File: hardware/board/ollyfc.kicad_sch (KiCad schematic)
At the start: 84 parts, among them CN1 20021521-00010T1LF, J1 Conn_01x04, J3 Conn_01x07, J4 Conn_01x06, Q2 MMBT3904, Q3 MMBT3904, SW1 MODE1, SW2 SW_Push, SW5 MODE1, U3 STM32F411RETx, U6 W25Q128JVS, X1 X322516MLB4SI

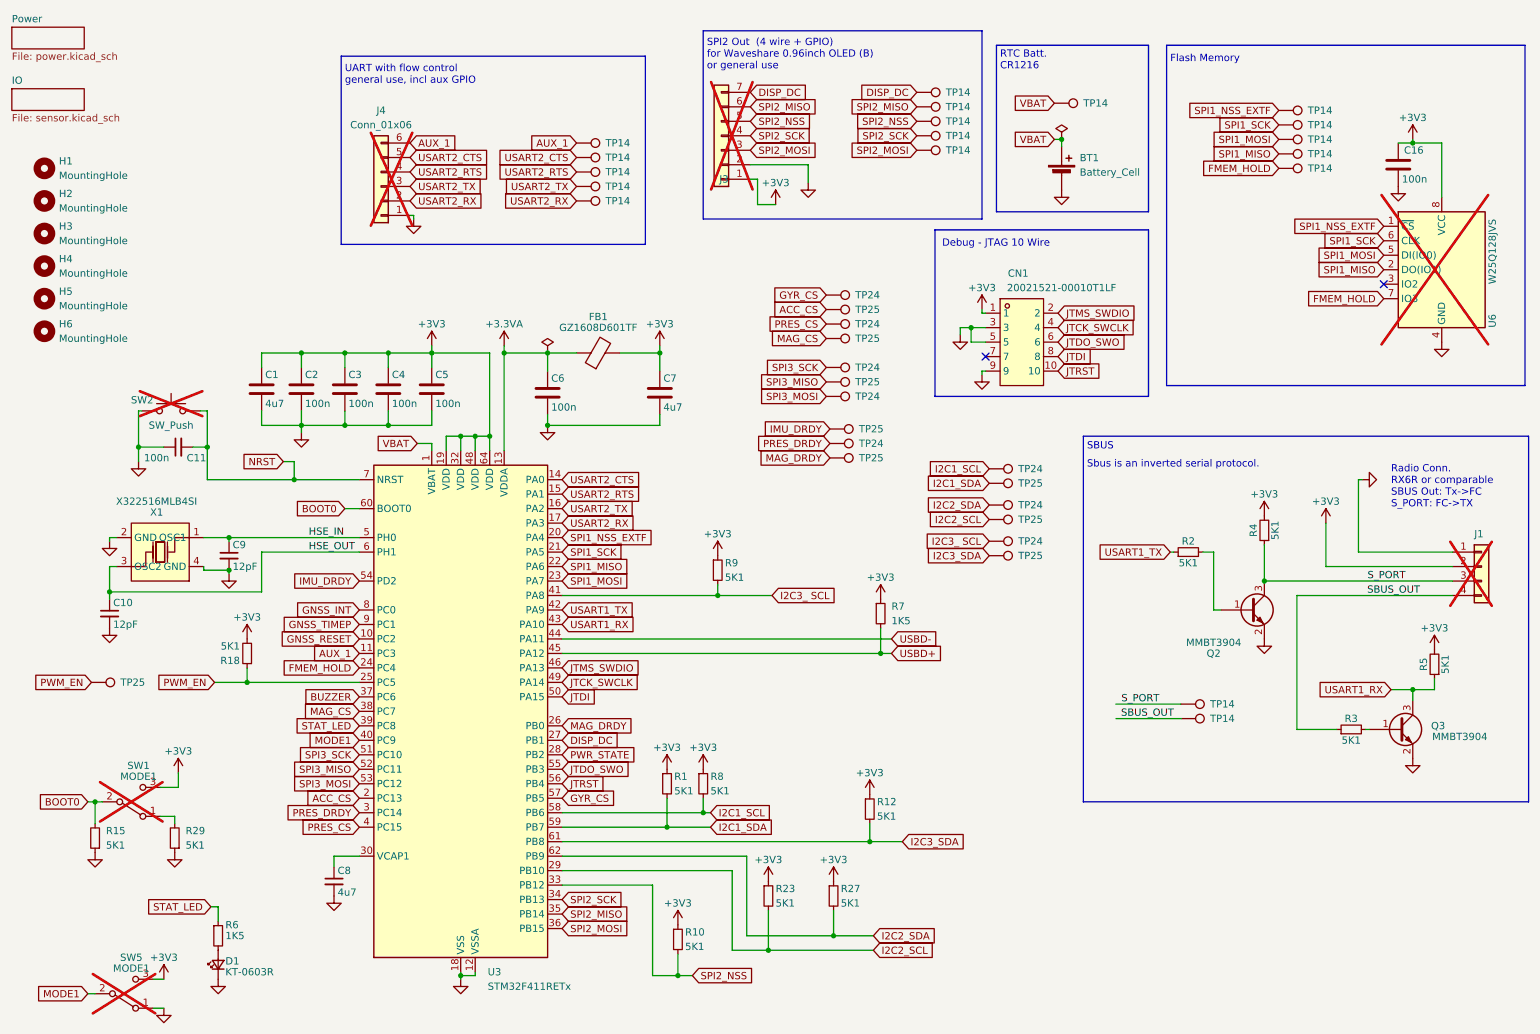
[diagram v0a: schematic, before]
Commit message: dead-end board files
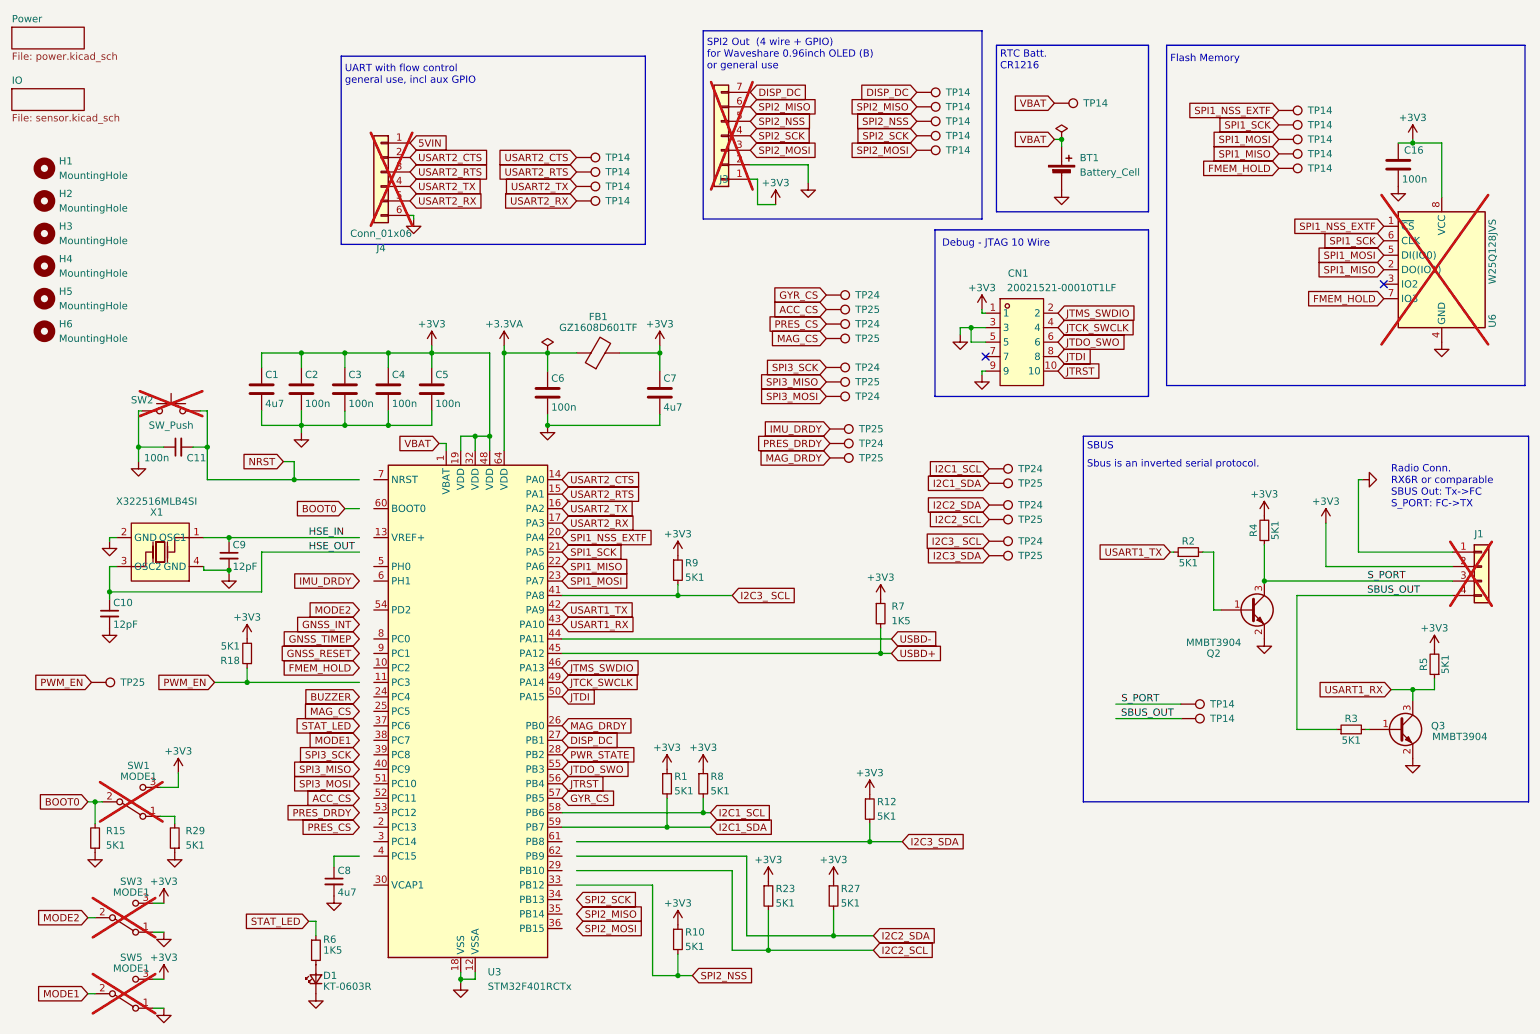
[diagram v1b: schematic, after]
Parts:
- removed TP14: TestPoint, TestPoint:TestPoint_Pad_D1.0mm, symbol Connector:TestPoint
- removed U3: STM32F411RETx, Package_QFP:LQFP-64_10x10mm_P0.5mm, symbol MCU_ST_STM32F4:STM32F411RETx
- added SW3: MODE1, Button_Switch_SMD:SW_SPDT_PCM12, symbol Switch:SW_SPDT
- added U3: STM32F401RCTx, Package_QFP:LQFP-64_10x10mm_P0.5mm, symbol MCU_ST_STM32F4:STM32F401RCTx
- J1: footprint Connector_JST:JST_PH_B4B-PH-K_1x04_P2.00mm_Vertical -> Connector_JST:JST_GH_BM04B-GHS-TBT_1x04-1MP_P1.25mm_Vertical
- J3: footprint Connector_JST:JST_PH_B7B-PH-K_1x07_P2.00mm_Vertical -> Connector_JST:JST_GH_BM07B-GHS-TBT_1x07-1MP_P1.25mm_Vertical
- J4: footprint Connector_JST:JST_PH_B6B-PH-K_1x06_P2.00mm_Vertical -> Connector_JST:JST_GH_SM06B-GHS-TB_1x06-1MP_P1.25mm_Horizontal
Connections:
- net AUX_1 is gone; now on net GND: J4.6 (Pin_6)
- net +3.3VA: now also U3.64 (VDD)
- net +3V3: now also SW3.3 (C), U3.19 (VDD), U3.32 (VDD), U3.48 (VDD)
- net DISP_DC: now also U3.27 (PB1)
- net GND: now also SW3.1 (A), U3.12 (VSSA), U3.18 (VSS), U3.31 (VSS), U3.47 (VSS), U3.63 (VSS); no longer J4.1 (Pin_1)
- net GYR_CS: now also U3.57 (PB5)
- net I2C1_SCL: now also U3.58 (PB6)
- net I2C1_SDA: now also U3.59 (PB7)
- net I2C3_ SCL: now also U3.41 (PA8)
- net JTCK_SWCLK: now also U3.49 (PA14)
- net JTDI: now also U3.50 (PA15)
- net JTDO_SWO: now also U3.55 (PB3)
- net JTMS_SWDIO: now also U3.46 (PA13)
- net JTRST: now also U3.56 (PB4)
- net MAG_DRDY: now also U3.26 (PB0)
- net PWR_STATE: now also U3.28 (PB2)
- net SPI1_MISO: now also U3.22 (PA6)
- net SPI1_MOSI: now also U3.23 (PA7)
- net SPI1_NSS_EXTF: now also U3.20 (PA4)
- net SPI1_SCK: now also U3.21 (PA5)
- net USART1_RX: now also U3.43 (PA10)
- net USART1_TX: now also U3.42 (PA9)
- net USART2_CTS: now also J4.2 (Pin_2), U3.14 (PA0); no longer J4.5 (Pin_5)
- net USART2_RTS: now also J4.3 (Pin_3), U3.15 (PA1); no longer J4.4 (Pin_4)
- net USART2_RX: now also J4.5 (Pin_5), U3.17 (PA3); no longer J4.2 (Pin_2)
- net USART2_TX: now also J4.4 (Pin_4), U3.16 (PA2); no longer J4.3 (Pin_3)
- net USBD+: now also U3.45 (PA12)
- net USBD-: now also U3.44 (PA11)
- net VBAT: now also U3.1 (VBAT)
- new net 5VIN: J4.1 (Pin_1)
- new net MODE2: SW3.2 (B)
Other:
- moved on the sheet: D1, J4, R6, R9
